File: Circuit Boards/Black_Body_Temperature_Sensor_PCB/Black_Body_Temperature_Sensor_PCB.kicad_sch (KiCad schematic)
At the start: 0 parts

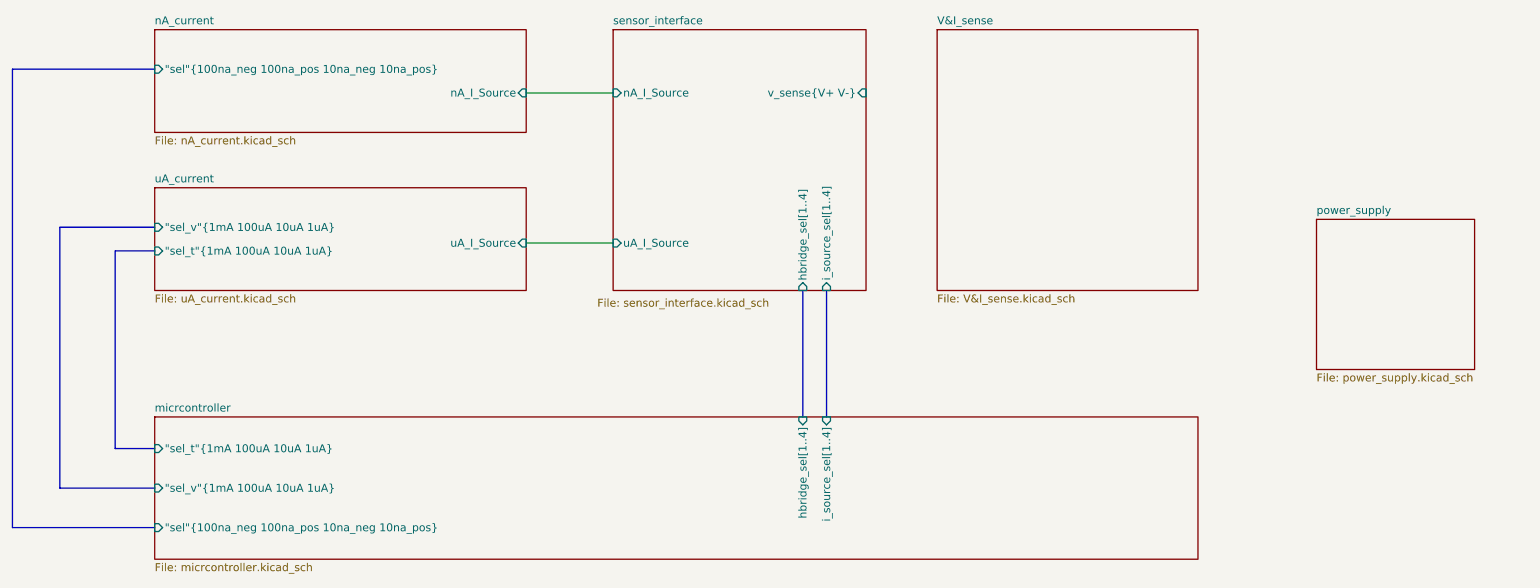
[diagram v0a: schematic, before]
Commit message: Schematic ready for review
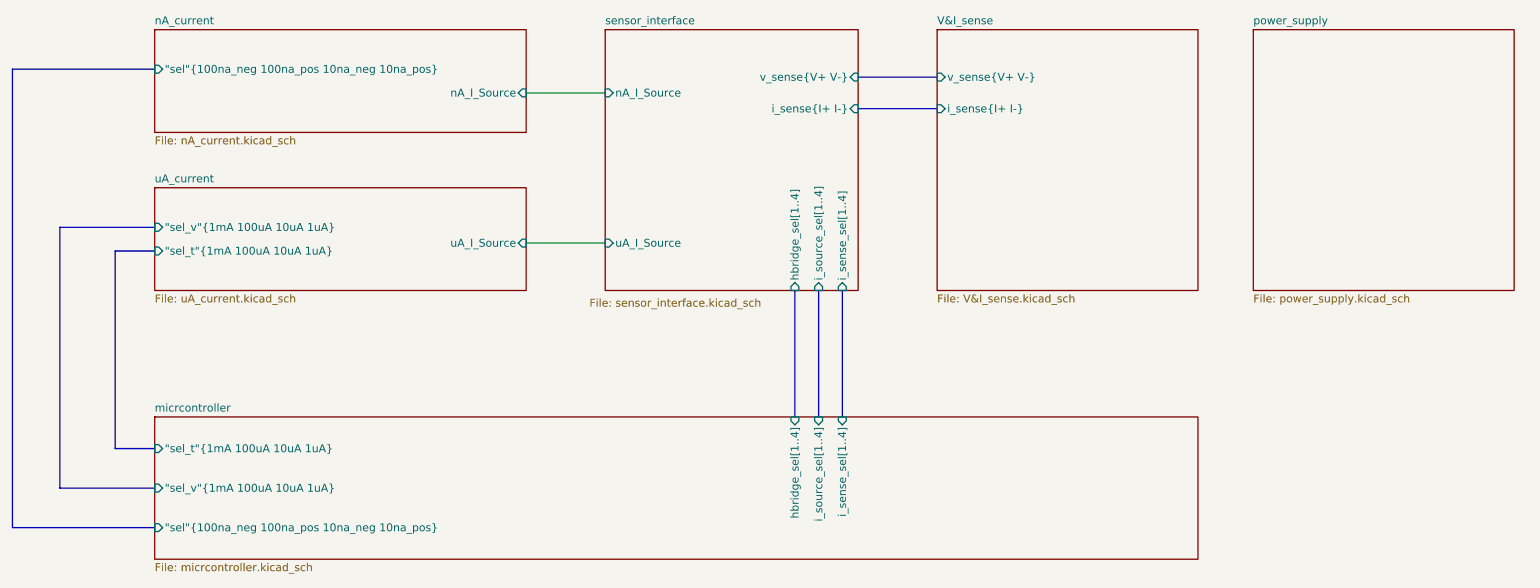
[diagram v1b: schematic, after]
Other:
- sheet V&I_sense ports: added i_sense{I+ I-}, v_sense{V+ V-}; removed none
- sheet micrcontroller ports: added i_sense_sel[1..4]; removed none
- sheet sensor_interface ports: added i_sense_sel[1..4], i_sense{I+ I-}; removed none
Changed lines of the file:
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@@
 	(bus
 		(pts
-			(xy 162.56 80.01) (xy 162.56 100.33)
+			(xy 167.64 50.8) (xy 180.34 50.8)
+		)
+		(stroke
+			(width 0)
+			(type default)
+		)
+	)
+	(bus
+		(pts
+			(xy 161.29 80.01) (xy 161.29 100.33)
 		)
 		(stroke
@@
 	(wire
 		(pts
-			(xy 114.3 48.26) (xy 128.27 48.26)
+			(xy 114.3 48.26) (xy 127 48.26)
 		)
 		(stroke
@@
 		)
 	)
+	(bus
+		(pts
+			(xy 167.64 45.72) (xy 180.34 45.72)
+		)
+		(stroke
+			(width 0)
+			(type default)
+		)
+	)
+	(bus
+		(pts
+			(xy 165.1 80.01) (xy 165.1 100.33)
+		)
+		(stroke
+			(width 0)
+			(type default)
+		)
+	)
 	(wire
 		(pts
-			(xy 114.3 72.39) (xy 128.27 72.39)
+			(xy 114.3 72.39) (xy 127 72.39)
 		)
 		(stroke
@@
 	(bus
 		(pts
-			(xy 158.75 80.01) (xy 158.75 100.33)
+			(xy 157.48 80.01) (xy 157.48 100.33)
 		)
 		(stroke
@@
 		)
 		(pin "hbridge_sel[1..4]" input
-			(at 158.75 100.33 90)
+			(at 157.48 100.33 90)
 			(effects
 				(font
@@
 		)
 		(pin "i_source_sel[1..4]" input
-			(at 162.56 100.33 90)
+			(at 161.29 100.33 90)
 			(effects
 				(font
@@
 				)
 				(justify left)
+			)
+		)
+		(pin "i_sense_sel[1..4]" input
+			(at 165.1 100.33 90)
+			(effects
+				(font
+					(size 1.27 1.27)
+				)
+				(justify right)
 			)
 		)
@@
 			(project "Black_Body_Temperature_Sensor_PCB"
 				(path "/e46fba8d-0294-4f4f-927d-8614bb9d51d3"
-					(page "5")
+					(page "7")
 				)
 			)
@@
 	)
 	(sheet
-		(at 128.27 38.1)
+		(at 127 38.1)
 		(size 40.64 41.91)
 		(exclude_from_sim no)
@@
 		)
 		(property "Sheetname" "sensor_interface"
-			(at 128.27 37.3884 0)
+			(at 127 37.3884 0)
 			(show_name no)
 			(do_not_autoplace no)
@@
 		)
 		(property "Sheetfile" "sensor_interface.kicad_sch"
-			(at 125.73 81.28 0)
+			(at 124.46 81.28 0)
 			(show_name no)
 			(do_not_autoplace no)
@@
 		)
 		(pin "v_sense{V+ V-}" input
-			(at 168.91 48.26 0)
+			(at 167.64 45.72 0)
 			(effects
 				(font
@@
 		)
 		(pin "uA_I_Source" input
-			(at 128.27 72.39 180)
+			(at 127 72.39 180)
 			(effects
 				(font
@@
 		)
 		(pin "nA_I_Source" input
-			(at 128.27 48.26 180)
+			(at 127 48.26 180)
 			(effects
 				(font
@@
 		)
 		(pin "i_source_sel[1..4]" input
-			(at 162.56 80.01 270)
+			(at 161.29 80.01 270)
 			(effects
 				(font
@@
 		)
 		(pin "hbridge_sel[1..4]" input
-			(at 158.75 80.01 270)
+			(at 157.48 80.01 270)
+			(effects
+				(font
+					(size 1.27 1.27)
+				)
+				(justify left)
+			)
+		)
+		(pin "i_sense{I+ I-}" input
+			(at 167.64 50.8 0)
+			(effects
+				(font
+					(size 1.27 1.27)
+				)
+				(justify right)
+			)
+		)
+		(pin "i_sense_sel[1..4]" input
+			(at 165.1 80.01 270)
 			(effects
 				(font
@@
 			(project "Black_Body_Temperature_Sensor_PCB"
 				(path "/e46fba8d-0294-4f4f-927d-8614bb9d51d3"
-					(page "6")
+					(page "4")
 				)
 			)
@@
 			)
 		)
+		(pin "v_sense{V+ V-}" input
+			(at 180.34 45.72 180)
+			(effects
+				(font
+					(size 1.27 1.27)
+				)
+				(justify left)
+			)
+		)
+		(pin "i_sense{I+ I-}" input
+			(at 180.34 50.8 180)
+			(effects
+				(font
+					(size 1.27 1.27)
+				)
+				(justify left)
+			)
+		)
 		(instances
 			(project "Black_Body_Temperature_Sensor_PCB"
 				(path "/e46fba8d-0294-4f4f-927d-8614bb9d51d3"
-					(page "4")
+					(page "5")
 				)
 			)
@@
 	)
 	(sheet
-		(at 241.3 68.58)
-		(size 25.4 24.13)
+		(at 231.14 38.1)
+		(size 41.91 41.91)
 		(exclude_from_sim no)
 		(in_bom yes)
@@
 		)
 		(property "Sheetname" "power_supply"
-			(at 241.3 67.8684 0)
+			(at 231.14 37.3884 0)
 			(show_name no)
 			(do_not_autoplace no)
@@
 		)
 		(property "Sheetfile" "power_supply.kicad_sch"
-			(at 241.3 93.2946 0)
+			(at 231.14 80.5946 0)
 			(show_name no)
 			(do_not_autoplace no)
@@
 			(project "Black_Body_Temperature_Sensor_PCB"
 				(path "/e46fba8d-0294-4f4f-927d-8614bb9d51d3"
-					(page "7")
-				)
-			)
+					(page "6")
+				)
+			)
